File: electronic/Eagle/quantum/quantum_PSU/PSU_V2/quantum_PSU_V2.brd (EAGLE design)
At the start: 140 x 110 mm, 30 parts, among them J1 90814-0204, J2 90814-0204, J3 PF0030_PC, U1 7815, U2 7812, U3 7915, U4 7805, U5 LD1117AV33

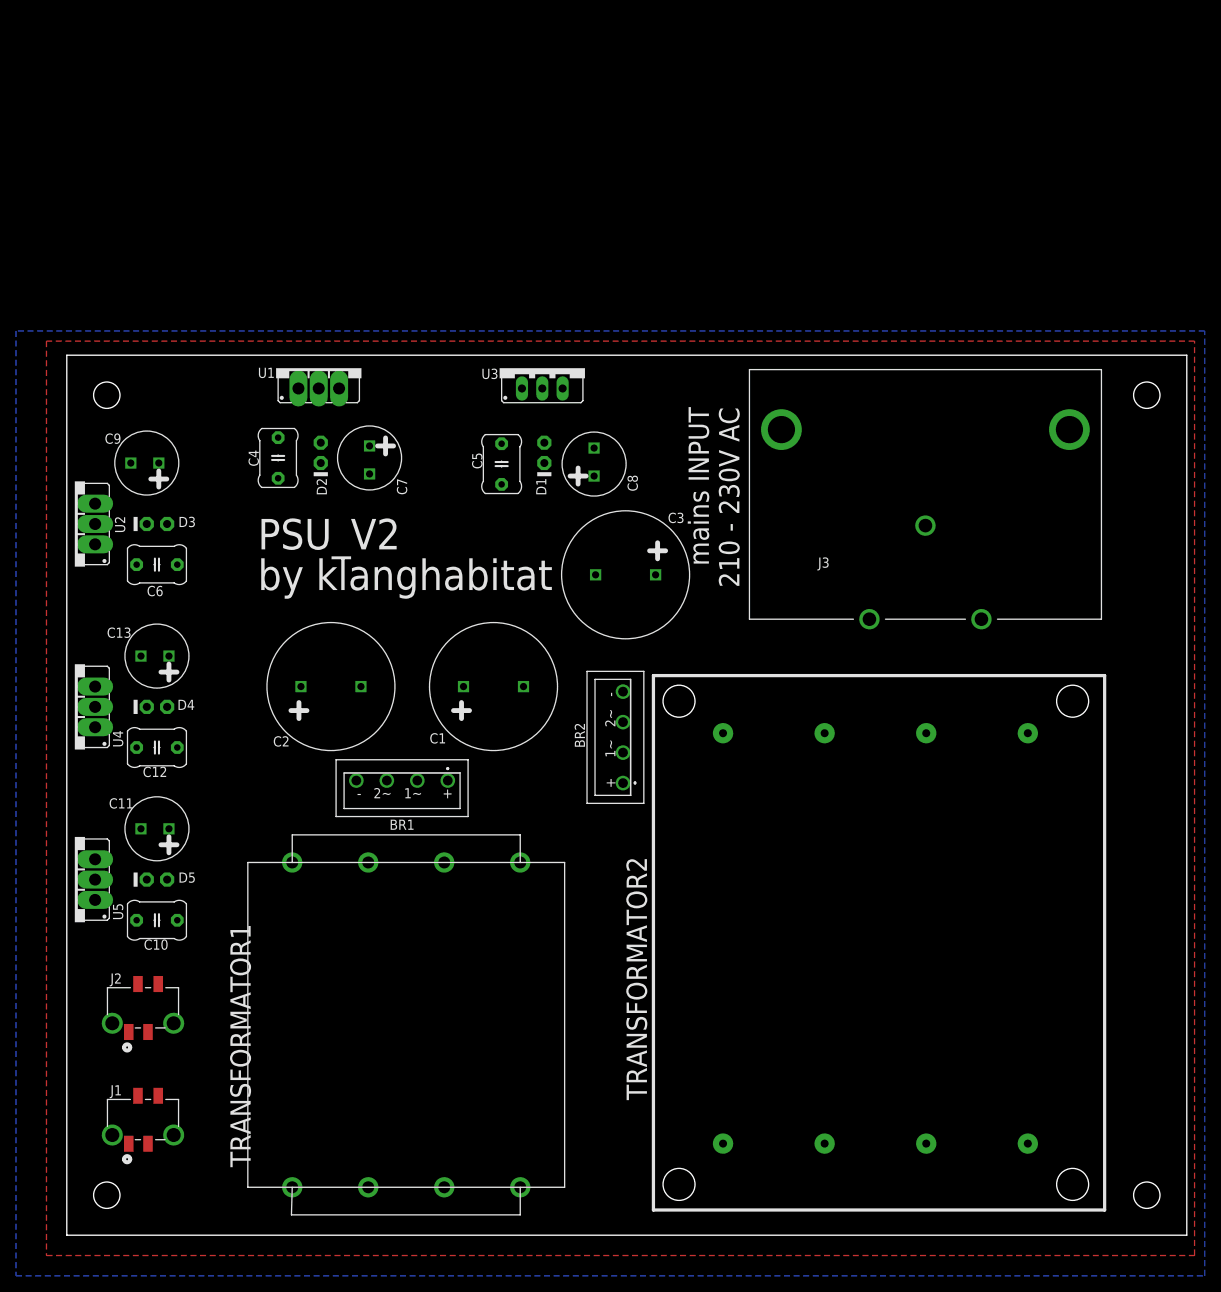
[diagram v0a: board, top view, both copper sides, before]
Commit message: progress PSU_V2
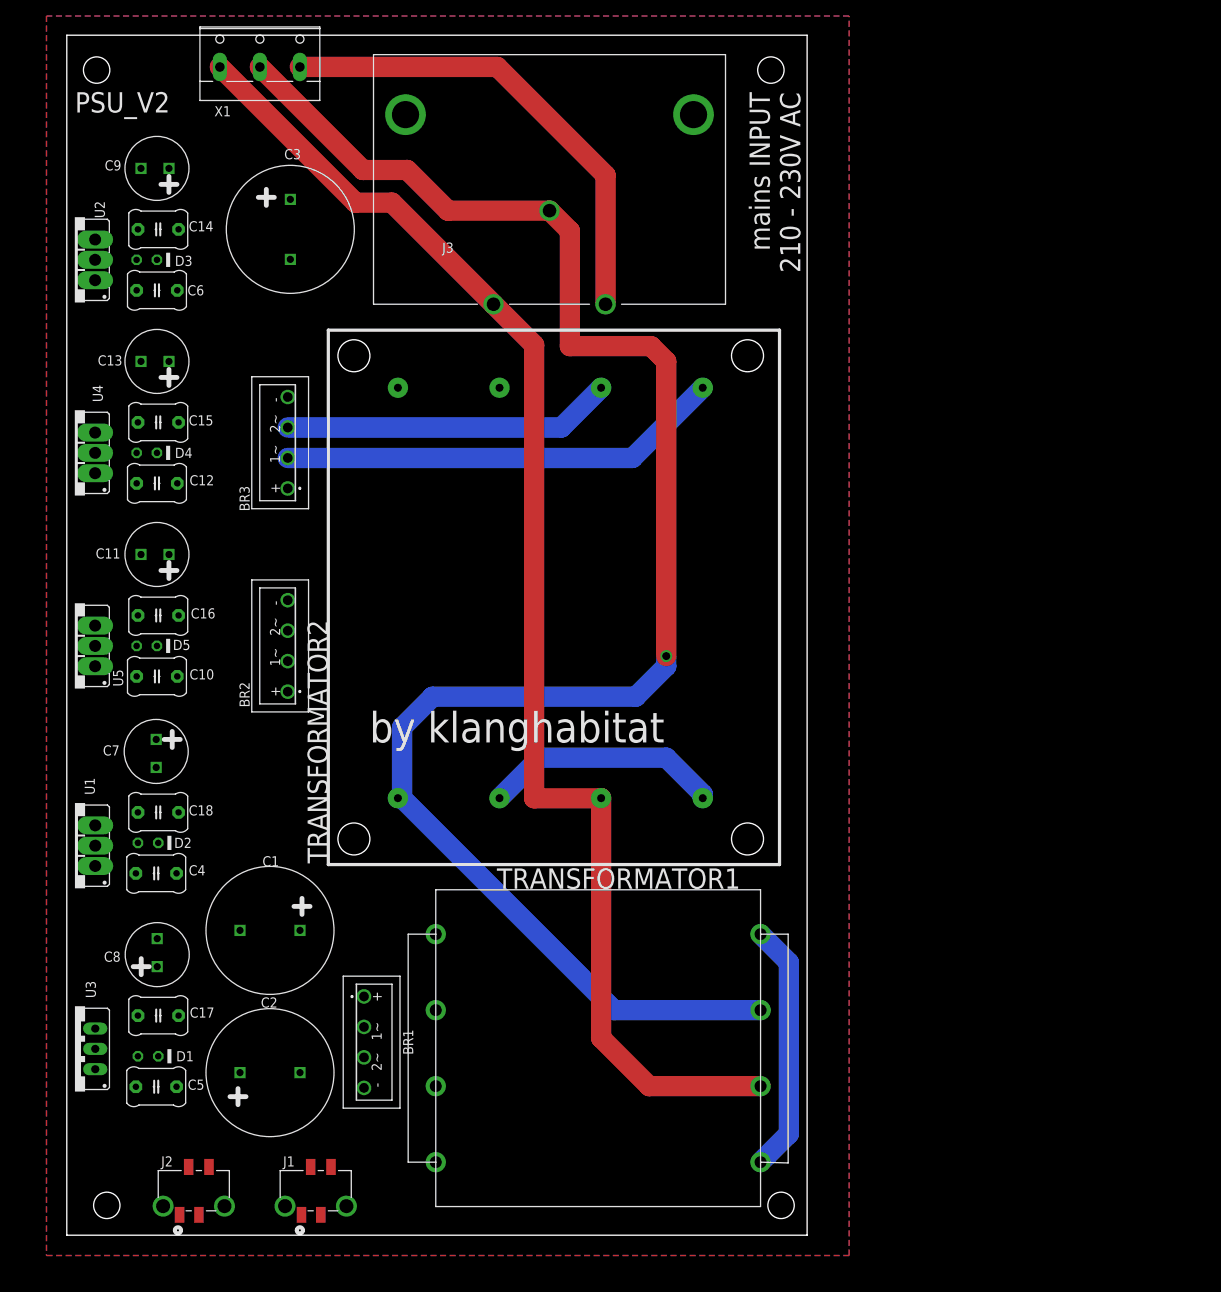
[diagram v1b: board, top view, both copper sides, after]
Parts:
- added BR3: BRIDGE_RECTIFIER, passive components:KBP308G
- added C14, C15, C16, C17, C18: 100 nF, passive components:C5MM
- added X1: (no value), electro_mechanical:W237-103
- moved U3 103.2 mm to (1.02, 23.3), turned to 90 degrees
- moved D1 92.0 mm to (8.89, 22.4), turned to 180 degrees
- moved C5 88.5 mm to (9.91, 18.6), turned to 0 degrees
- moved C8 82.1 mm to (11.3, 35.1)
- moved U1 67.0 mm to (1.02, 48.7), turned to 90 degrees
- moved J3 61.3 mm to (53.3, 116.4)
- moved C3 60.2 mm to (27.9, 125.7), turned to 270 degrees
- moved TRANSFORMATOR2 59.3 mm to (85.1, 49.5)
- moved C4 55.7 mm to (9.91, 45.2), turned to 0 degrees
- moved D2 55.0 mm to (8.89, 49.0), turned to 180 degrees
- moved TRANSFORMATOR1 49.3 mm to (90.2, 43.2), turned to 180 degrees
- moved C2 48.9 mm to (25.4, 20.3)
- moved C7 45.4 mm to (11.2, 60.5)
- moved BR2 43.4 mm to (26.7, 73.7)
- moved C1 41.3 mm to (25.4, 38.1), turned to 180 degrees
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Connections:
- removed net N$1: BR2.2, TRANSFORMATOR2.P$6, TRANSFORMATOR2.P$7
- removed net N$13: BR1.3, TRANSFORMATOR1.P$5
- new net N$4: TRANSFORMATOR1.P$1, TRANSFORMATOR1.P$4
- new net N$5: TRANSFORMATOR2.P$1, TRANSFORMATOR2.P$4
- new net N$6: TRANSFORMATOR2.P$8
- net +12V_OUT: now also C14.1
- net +15V_OUT: now also C18.1
- net +3V3_OUT: now also C16.1
- net +5V_OUT: now also C15.1
- net -15V_OUT: now also C17.2
- net AGND: now also C17.1, C18.2, TRANSFORMATOR1.P$5; no longer TRANSFORMATOR1.P$6
- net CHASSIS: now also X1.3
- net DGND: now also BR3.4, C14.2, C15.2, C16.2
- net N$10: now also BR3.2, TRANSFORMATOR2.P$5; no longer TRANSFORMATOR2.P$2, TRANSFORMATOR2.P$4
- net N$2: now also BR3.1
- net N$3: now also BR1.3, TRANSFORMATOR1.P$6; no longer BR2.3, TRANSFORMATOR2.P$5, TRANSFORMATOR2.P$8
- net N$7: now also BR3.3, TRANSFORMATOR2.P$6; no longer TRANSFORMATOR1.P$2, TRANSFORMATOR1.P$4
- net N$8: now also X1.2
- net N$9: now also TRANSFORMATOR1.P$2, TRANSFORMATOR2.P$2, X1.1; no longer TRANSFORMATOR1.P$1, TRANSFORMATOR2.P$1
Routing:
- net N$8: track 0.00 -> 214.0 mm, vias 0 -> 1
- net N$9: track 0.00 -> 171.1 mm
- net CHASSIS: track 0.00 -> 59.9 mm
- net N$10: track 0.00 -> 55.5 mm
- net N$7: track 0.00 -> 41.2 mm
- net N$4: track 0.00 -> 31.4 mm
- net N$5: track 0.00 -> 29.9 mm
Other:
- board size 140 x 110 mm -> 92.5 x 150 mm
